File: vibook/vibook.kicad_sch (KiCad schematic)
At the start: 54 parts, among them IC3 STLQ020C33R, J1 Conn_ARM_JTAG_SWD_10, J2 6861XX148922_686112148922, J3 6861XX148922_686112148922, SW3 SW_Push, U2 STM32L011K4Ux, U3 MPR121QR2, U5 MPR121QR2, U6 DFR0299

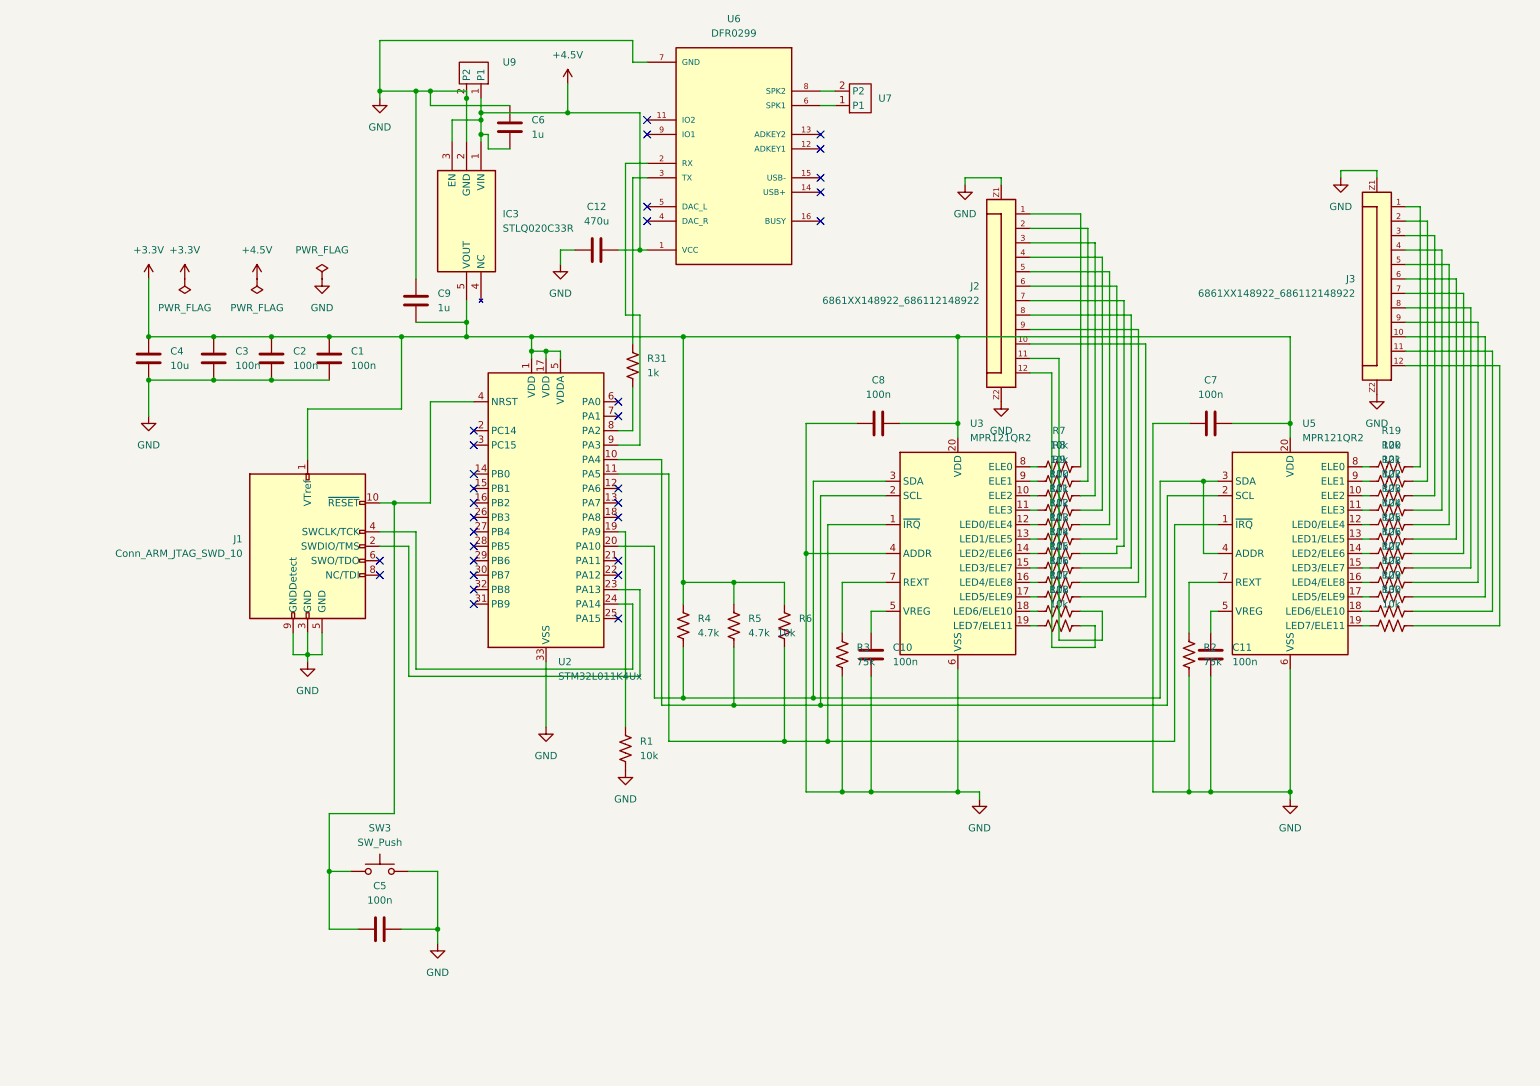
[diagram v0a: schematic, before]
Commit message: updated schematic
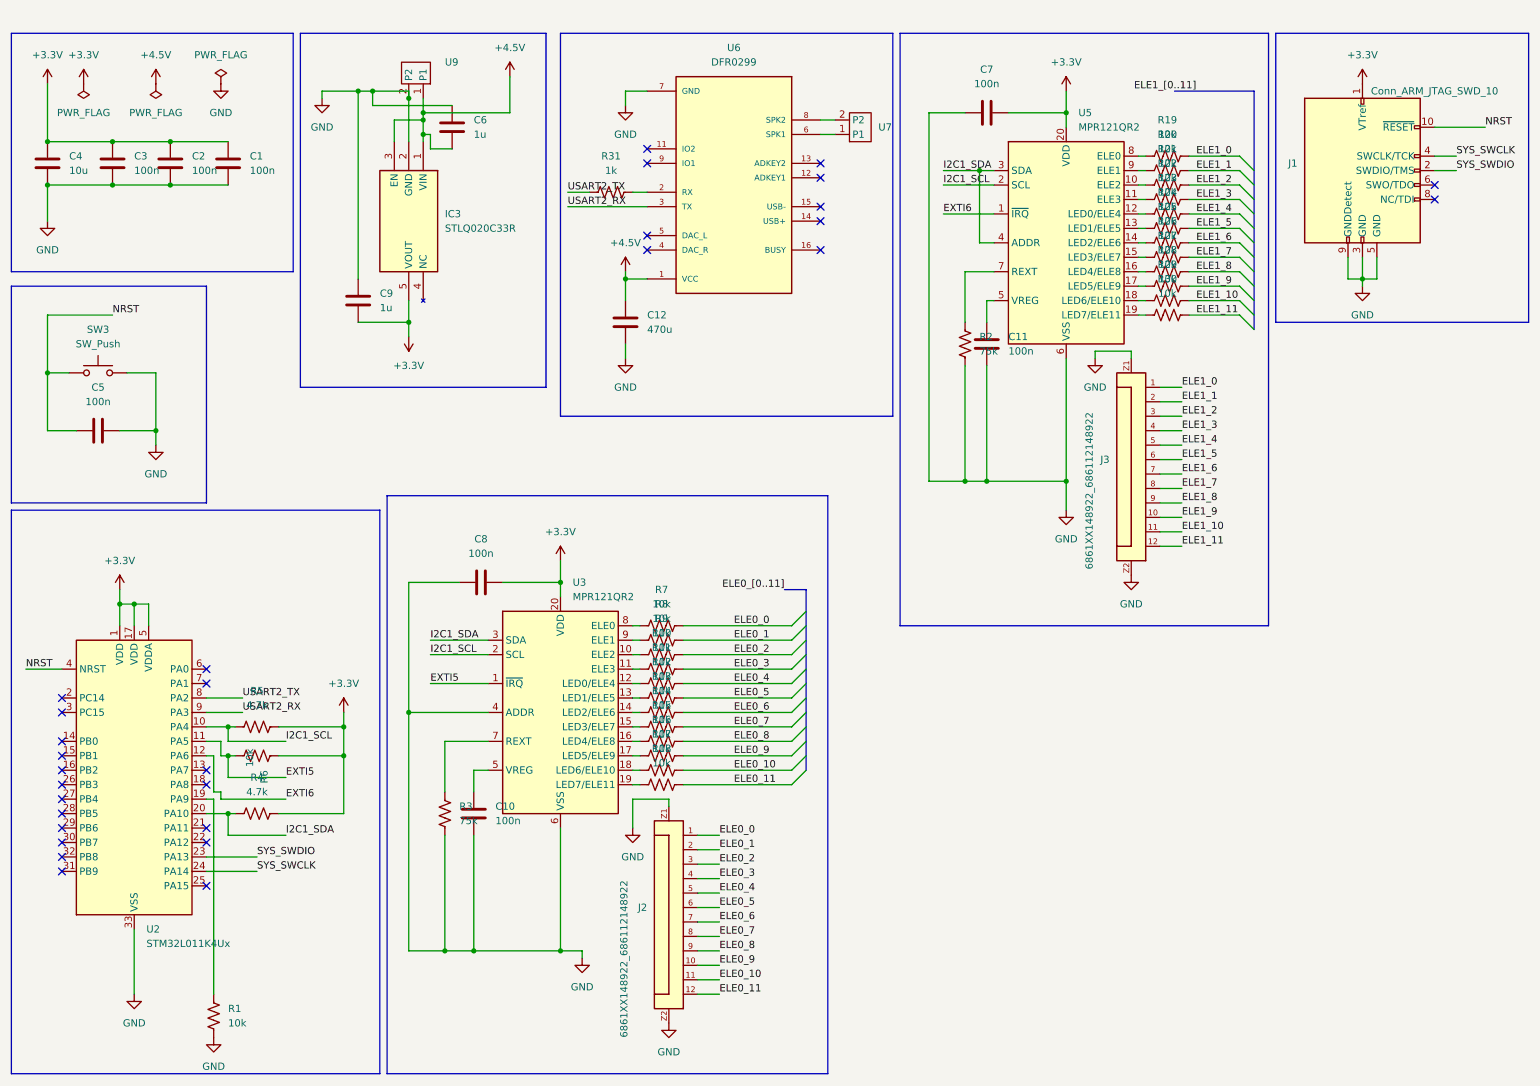
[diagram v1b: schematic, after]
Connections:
- net +3.3V: now also R4.2, R5.2; no longer R4.1, R5.1
- net ELE1_4: now reaches J3.5, R23.2
- net ELE1_8: now reaches J3.9, R27.2
- net EXTI5: now reaches R6.2, U2.11 (PA5), U3.1 (~{IRQ})
- net EXTI5: no longer U5.1 (~{IRQ})
- net I2C1_SCL: now reaches U2.10 (PA4), U3.2 (SCL), U5.2 (SCL)
- net I2C1_SCL: now also R5.1; no longer R5.2
- net I2C1_SDA: now reaches U2.20 (PA10), U3.3 (SDA), U5.3 (SDA), U5.4 (ADDR)
- net I2C1_SDA: now also R4.1; no longer R4.2
- net ELE1_3: now reaches J3.4, R22.2
- net ELE1_6: now reaches J3.7, R25.2
- net ELE0_5: now reaches J2.6, R12.2
- net NRST: now reaches C5.1, J1.10 (~{RESET}), SW3.1, U2.4 (NRST)
- net ELE0_11: now reaches J2.12, R18.2
- net ELE1_2: now reaches J3.3, R21.2
- net ELE0_4: now reaches J2.5, R11.2
- net ELE0_2: now reaches J2.3, R9.2
- net ELE0_7: now reaches J2.8, R14.2
- net at U6.2 (RX): now also R31.2; no longer U2.9 (PA3)
- net USART2_RX: now reaches U6.3 (TX)
- net USART2_RX: now also U2.9 (PA3); no longer R31.1
- net USART2_TX: now reaches U2.8 (PA2)
- net USART2_TX: now also R31.1; no longer R31.2
- net ELE0_10: now reaches J2.11, R17.2
- net ELE1_0: now reaches J3.1, R19.2
- net ELE1_5: now reaches J3.6, R24.2
- net ELE0_9: now reaches J2.10, R16.2
- net EXTI6: now reaches U2.12 (PA6)
- net EXTI6: now also U5.1 (~{IRQ})
- net SYS_SWDIO: now reaches J1.2 (SWDIO/TMS), U2.23 (PA13)
- net SYS_SWCLK: now reaches J1.4 (SWCLK/TCK), U2.24 (PA14)
- net ELE0_0: now reaches J2.1, R7.2
- net ELE1_9: now reaches J3.10, R28.2
- net ELE1_10: now reaches J3.11, R29.2
- net ELE1_11: now reaches J3.12, R30.2
- net ELE1_1: now reaches J3.2, R20.2
- net ELE1_7: now reaches J3.8, R26.2
- net ELE0_6: now reaches J2.7, R13.2
- net ELE0_3: now reaches J2.4, R10.2
- net ELE0_1: now reaches J2.2, R8.2
- net ELE0_8: now reaches J2.9, R15.2
- no-connect marks 31 -> 30
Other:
- moved on the sheet: C1, C10, C11, C12, C2, C3, C4, C5, C6, C7, C8, C9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
